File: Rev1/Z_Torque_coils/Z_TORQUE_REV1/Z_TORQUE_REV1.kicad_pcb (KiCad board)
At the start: 4 copper layers, 95.9 x 90.2 mm, 50 parts, among them IC1 MPM3610AGQV-Z, J1 F3311A7H121014E200, J2 F3311A7H121014E200, Q1 BSS138, Q2 BSS138, Q3 MBT2222ADW1T1, Q4 BSS138, Q5 BSS138, Q6 MBT2222ADW1T1, U1 DRV8830DGQ

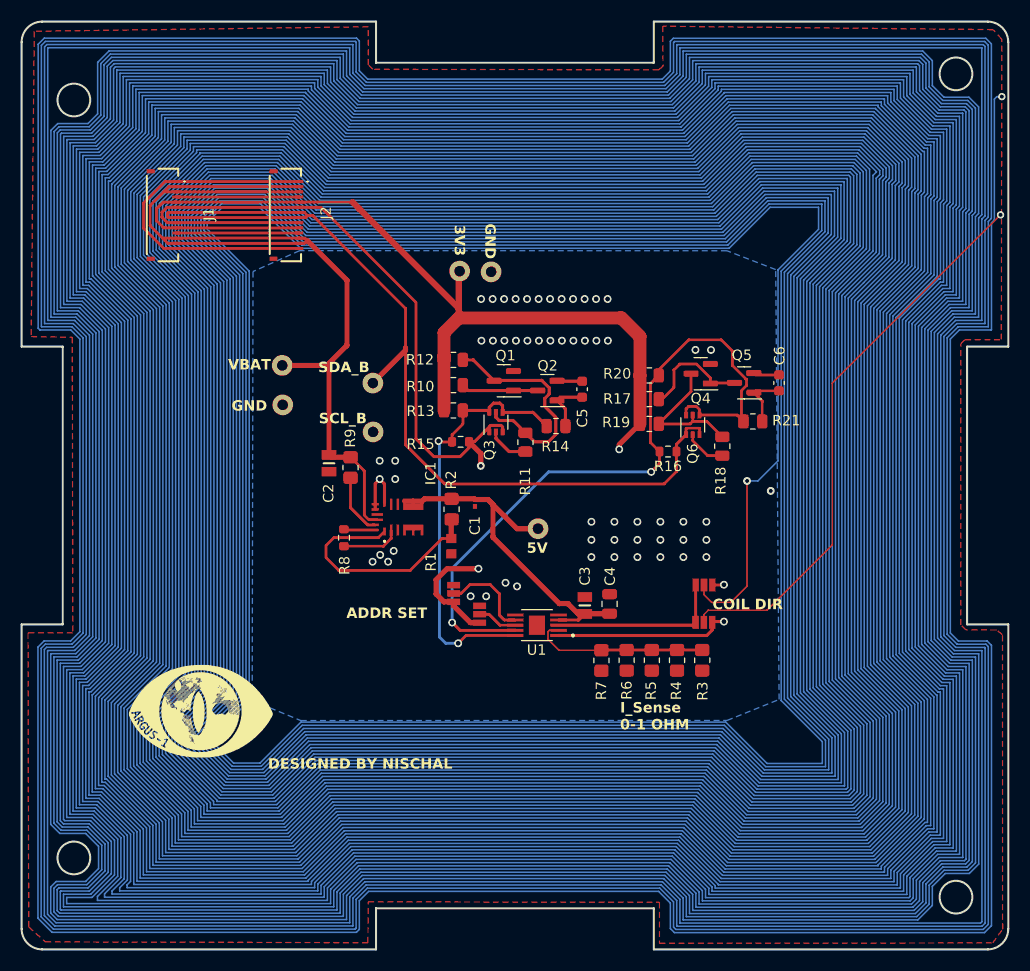
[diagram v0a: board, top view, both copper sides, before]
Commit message: made changes to step
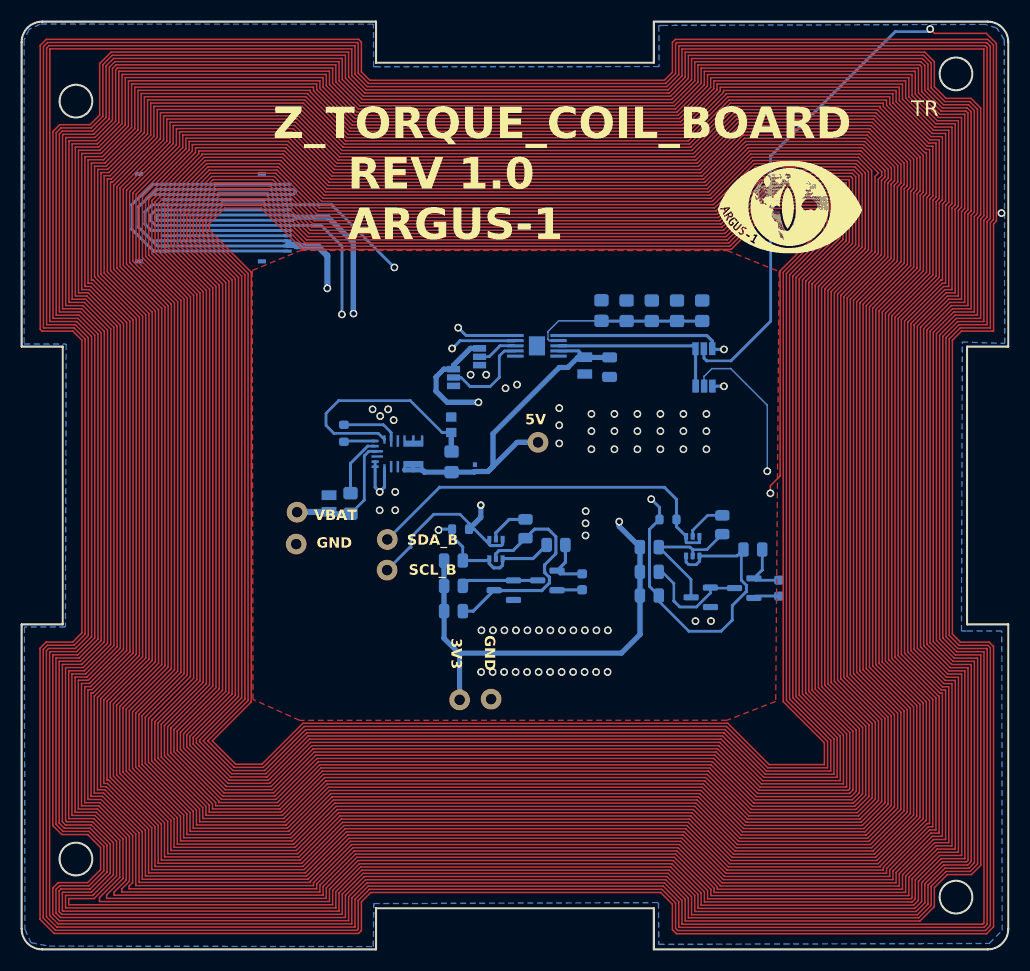
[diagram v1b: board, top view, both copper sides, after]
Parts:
- ., ? (x7): moved to F.Cu
- ., C1, C2, C3, C4, C5, C6, IC1, J1, J2, JP1, JP2, JP3, JP4, Q1, Q2, Q3, Q4, Q5, Q6, R1, R10, R11, R12, R13, R14, R15, R16, R17, R18, R19, R2, R20, R21, R3, R4, R5, R6, R7, R8, R9, U1: moved to B.Cu
- moved . 61.7 mm to (179.0, 65.6), turned to 0 degrees
- moved . 61.5 mm to (183.2, 114.6), turned to 180 degrees
- moved ? 41.7 mm to (147.1, 113.5)
- moved ? 41.5 mm to (150.2, 113.5)
- moved R7 34.0 mm to (160.9, 75.7), turned to 90 degrees
- moved R3 34.0 mm to (170.7, 75.7), turned to 90 degrees
- moved R4 34.0 mm to (168.2, 75.7), turned to 90 degrees
- moved R5 34.0 mm to (165.8, 75.7), turned to 90 degrees
- moved R6 34.0 mm to (163.3, 75.7), turned to 90 degrees
- moved U1 27.2 mm to (154.6, 79.1)
- moved JP3 26.6 mm to (170.8, 79.4)
- moved JP1 25.0 mm to (149.0, 80.2), turned to 90 degrees
- moved R12 24.4 mm to (146.5, 104.9)
- moved C3 23.3 mm to (159.3, 81.1), turned to 90 degrees
- moved C4 23.0 mm to (161.7, 81.2), turned to -90 degrees
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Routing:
- net +3.3V: track 126.2 -> 187.0 mm, vias 2 -> 3
- net GND: track 34.5 -> 54.6 mm, vias 56 -> 62
- net SCL1_b4iso: track 82.4 -> 101.7 mm, vias 1 -> 2
- net coils: track 50068.4 -> 50079.3 mm
- net SDA1_b4iso: track 94.0 -> 103.0 mm, vias 0 -> 1
- net VBATT: track 98.2 -> 104.2 mm, vias 0 -> 1
- net SCL_TORQUE: track 42.0 -> 43.3 mm
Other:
- outline, holes or cut-outs redrawn
- board text added: "1"
- board text added: "2"
- board text added: "A0"
- board text added: "A1"
- board text added: "TR"
